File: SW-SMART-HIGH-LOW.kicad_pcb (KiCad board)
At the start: 2 copper layers, 73 x 69 mm, 21 parts, among them IC1 MCP1416, J1 1 CTL IN, SW1 BTS50010-1TAD, SW2 VNB35N07xx-E

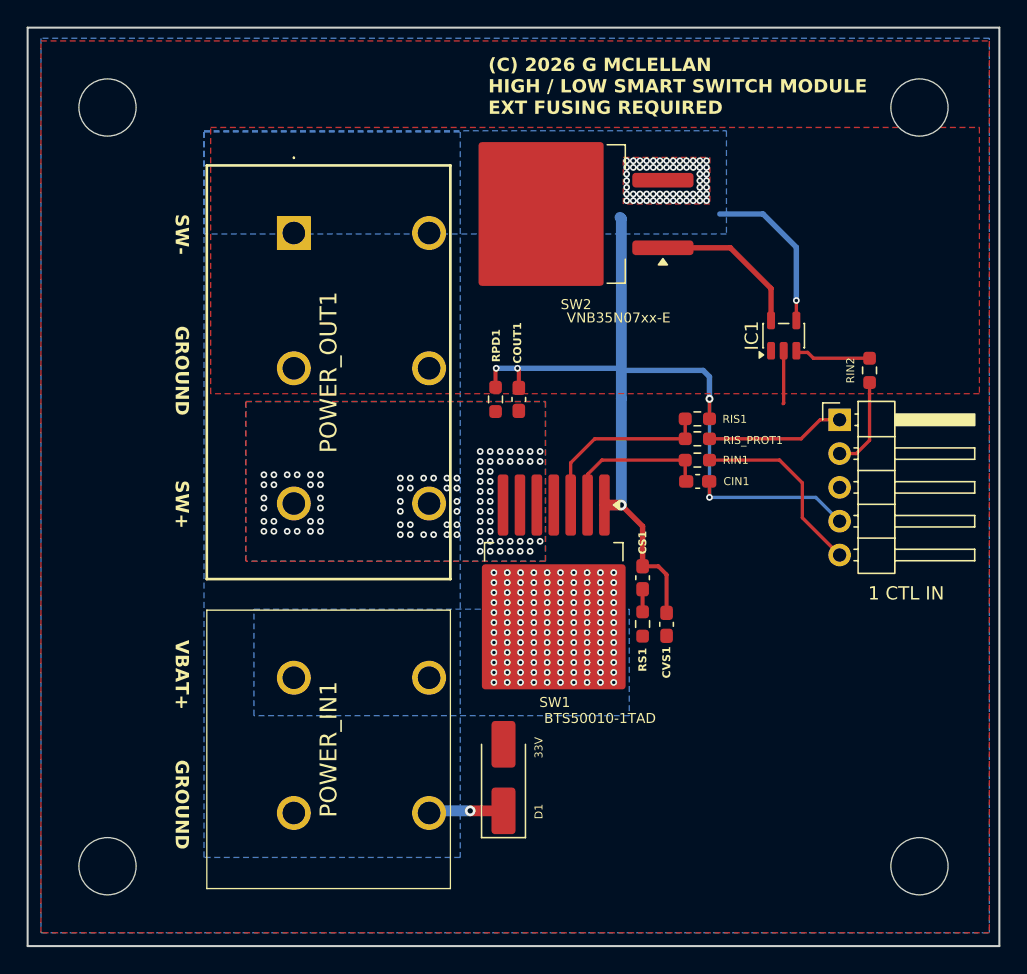
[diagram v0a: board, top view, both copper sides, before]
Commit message: fit a lot of stuff onto a small board
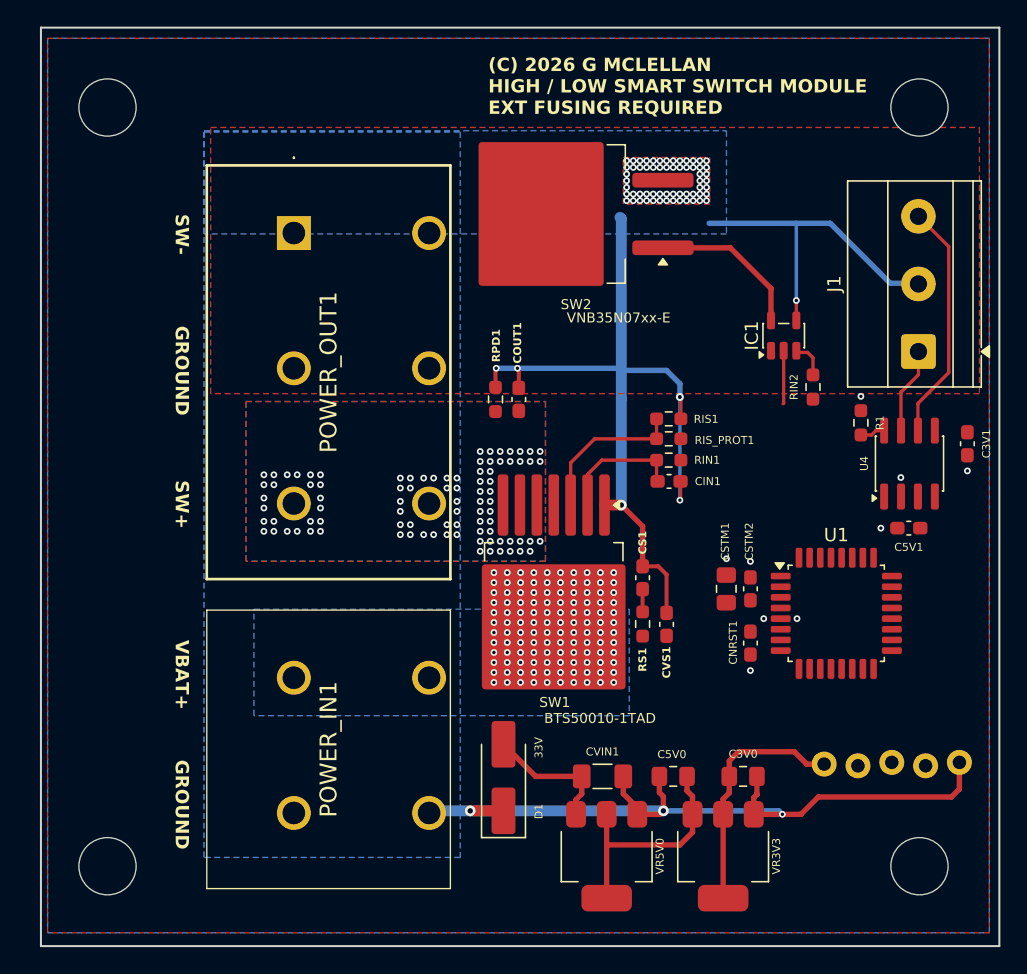
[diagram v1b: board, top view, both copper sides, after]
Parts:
- added C3V0: 10u, Capacitor_SMD:C_0805_2012Metric_Pad1.18x1.45mm_HandSolder, F.Cu at (133.8, 122.2)
- added C3V1: 100n, Capacitor_SMD:C_0603_1608Metric_Pad1.08x0.95mm_HandSolder, F.Cu at (150.6, 97.3)
- added C5V0: 10u, Capacitor_SMD:C_0805_2012Metric_Pad1.18x1.45mm_HandSolder, F.Cu at (128.5, 122.2)
- added C5V1: 100n, Capacitor_SMD:C_0603_1608Metric_Pad1.08x0.95mm_HandSolder, F.Cu at (146.2, 103.6)
- added CNRST1: 100n, Capacitor_SMD:C_0603_1608Metric_Pad1.08x0.95mm_HandSolder, F.Cu at (134.3, 112.2)
- added CSTM1: 4u7, Capacitor_SMD:C_0805_2012Metric_Pad1.18x1.45mm_HandSolder, F.Cu at (132.5, 108.2)
- added CSTM2: 100n, Capacitor_SMD:C_0603_1608Metric_Pad1.08x0.95mm_HandSolder, F.Cu at (134.3, 108.2)
- added CVIN1: 10u, Capacitor_SMD:C_1206_3216Metric_Pad1.33x1.80mm_HandSolder, F.Cu at (123.2, 122.2)
- added J2: SWLINK, PCM_SparkFun-Connector:1x05_P2.54mm_Locking, F.Cu at (139.8, 121.3)
- added R1: 10K, Resistor_SMD:R_0603_1608Metric_Pad0.98x0.95mm_HandSolder, F.Cu at (142.6, 95.7)
- added U1: STM32G0B1KBTx, Package_QFP:LQFP-32_7x7mm_P0.8mm, F.Cu at (140.8, 110.0)
- added U4: MCP2562-E-SN, Package_SO:SOIC-8_3.9x4.9mm_P1.27mm, F.Cu at (146.2, 98.8)
- added VR3V3: NCV1117ST33, PCM_SparkFun-Semiconductor-Standard:SOT-223-3_TabPin2, F.Cu at (132.2, 128.2)
- added VR5V0: NCV1117ST50, PCM_SparkFun-Semiconductor-Standard:SOT-223-3_TabPin2, F.Cu at (123.5, 128.2)
- J1: value 1 CTL IN -> H GND L; footprint Connector_PinHeader_2.54mm:PinHeader_1x05_P2.54mm_Horizontal -> TerminalBlock_Phoenix:TerminalBlock_Phoenix_MKDS-1,5-3-5.08_1x03_P5.08mm_Horizontal
- moved J1 7.83 mm to (146.9, 90.3), turned to 90 degrees
- moved RIN2 4.43 mm to (139.0, 93.0)
- moved CIN1 2.15 mm to (128.2, 100.1)
- moved RIN1 2.15 mm to (128.2, 98.5)
- moved RIS1 2.15 mm to (128.2, 95.4)
- moved RIS_PROT1 2.15 mm to (128.2, 96.9)
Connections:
- J1 pad 1: /SW1IS -> /CAN_H
- J1 pad 2: /LOW_IN -> GND
- J1 pad 3: unconnected-(J1-Pin_3-Pad3) -> /CAN_L
- RIN1 pad 1: /SW1IN -> unconnected-(RIN1-Pad1)
- RIN2 pad 1: /LOW_IN -> unconnected-(RIN2-Pad1)
- RIS_PROT1 pad 1: /SW1IS -> unconnected-(RIS_PROT1-Pad1)
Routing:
- net GND: track 92.6 -> 145.6 mm, vias 68 -> 79
- net +3.3V: track 0.00 -> 18.3 mm
- net /CAN_L: track 0.00 -> 18.0 mm
- net +5V: track 0.00 -> 17.5 mm
- net /SW1IN: track 14.3 -> 0.00 mm
- net /SW1IS: track 10.4 -> 0.00 mm
- net +12V: track 7.99 -> 17.9 mm
- net /LOW_IN: track 7.00 -> 0.00 mm
- net /CAN_H: track 0.00 -> 6.48 mm
- net Net-(IC1-IN): track 5.73 -> 2.75 mm
- net /SW1IS_PD: track 14.0 -> 11.9 mm
- net Net-(SW1-IN): track 11.7 -> 9.56 mm
- net Net-(U4-STBY): track 0.00 -> 1.88 mm
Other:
- board size 73 x 69 mm -> 72 x 69 mm
